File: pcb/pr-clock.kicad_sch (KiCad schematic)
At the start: 6 parts, among them J1 USB_C_Receptacle_USB2.0_16P, U1 TM1637_C2962580, U2 ESP32-C3-WROOM-02, U3 ME6211C33M5, U4 CH340C

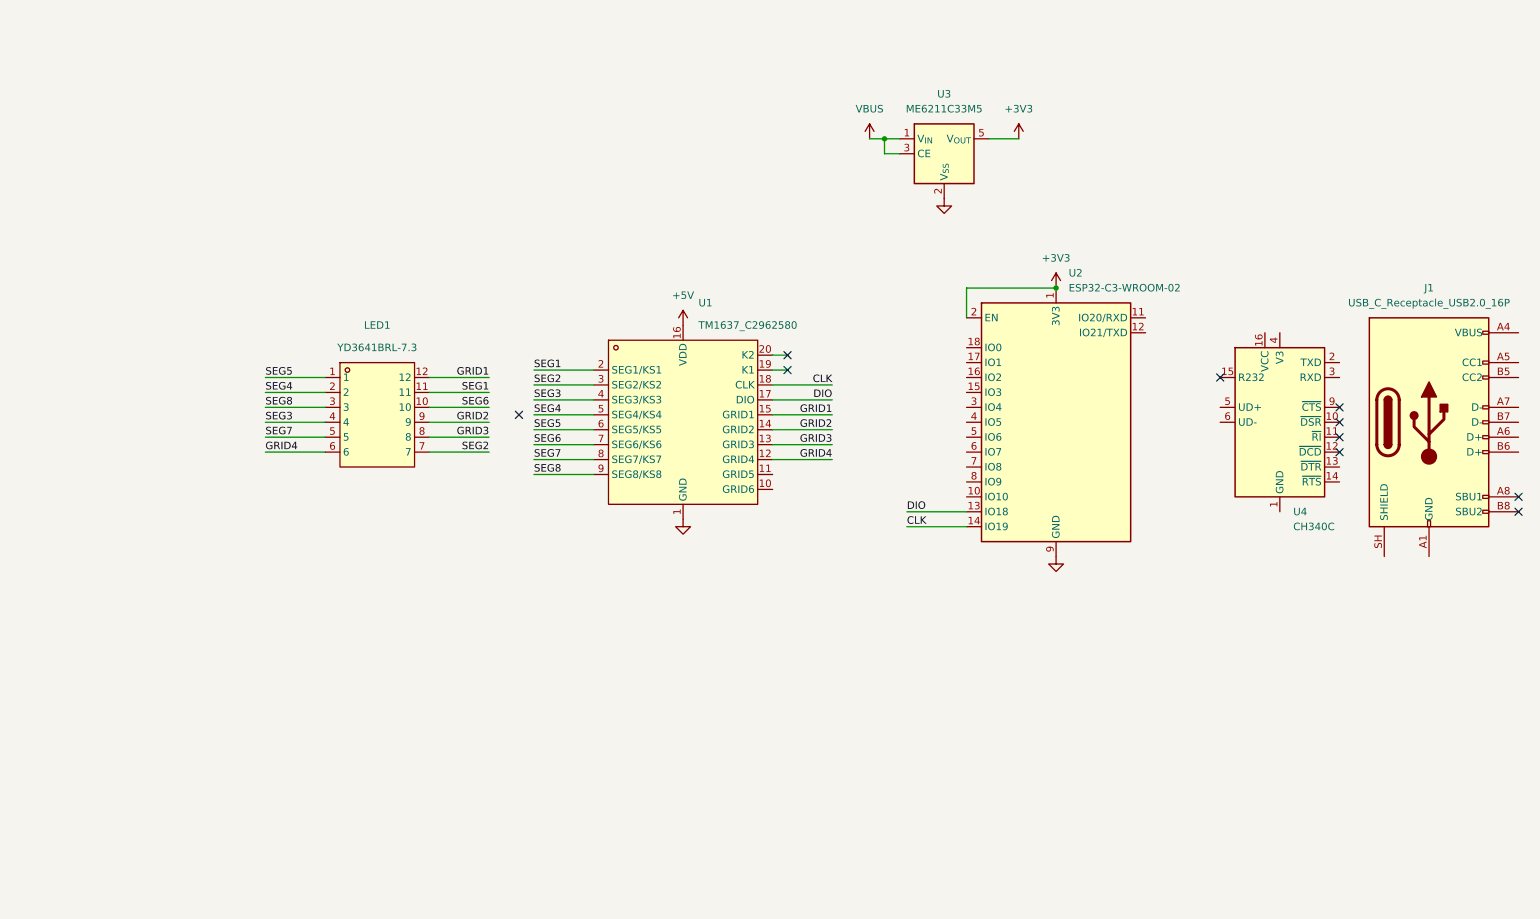
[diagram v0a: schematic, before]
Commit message: yay
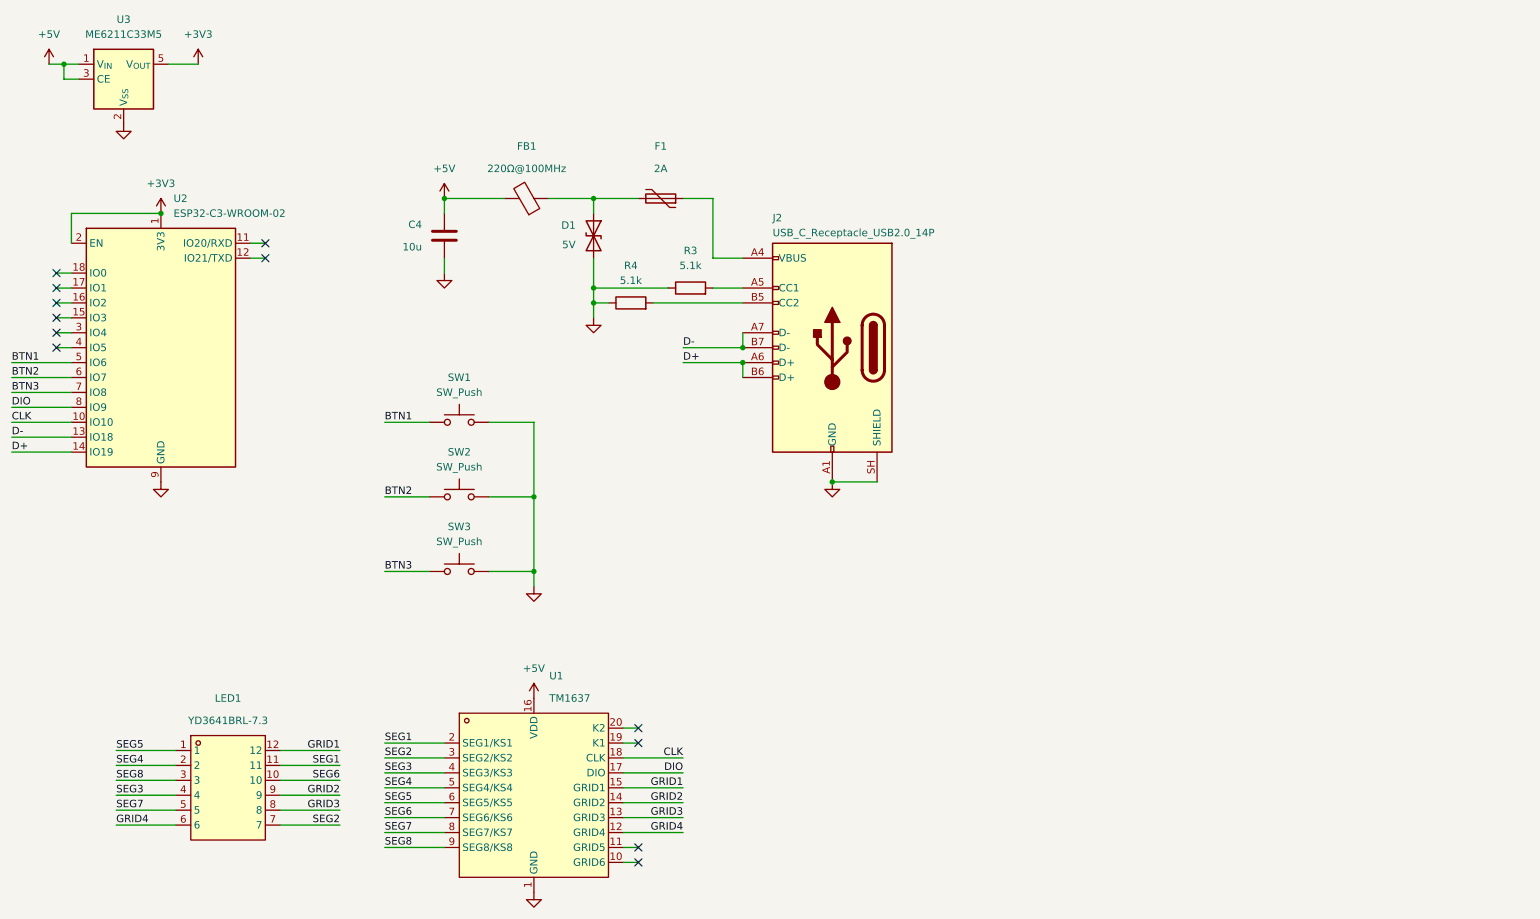
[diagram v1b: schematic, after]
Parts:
- removed J1: USB_C_Receptacle_USB2.0_16P, symbol Connector:USB_C_Receptacle_USB2.0_16P
- removed U4: CH340C, Package_SO:SOIC-16_3.9x9.9mm_P1.27mm, symbol Interface_USB:CH340C
- added C4: 10u, Capacitor_SMD:C_0603_1608Metric, symbol Device:C
- added D1: 5V, Diode_SMD:D_SOD-523, symbol Device:D_TVS
- added F1: 2A, Fuse:Fuse_1206_3216Metric, symbol Device:Polyfuse
- added FB1: 220Ω@100MHz, Resistor_SMD:R_0805_2012Metric_Pad1.20x1.40mm_HandSolder, symbol Device:FerriteBead
- added J2: USB_C_Receptacle_USB2.0_14P, easyeda2kicad:USB-C-SMD_TYPE-C-16PIN-2MD-073, symbol Connector:USB_C_Receptacle_USB2.0_14P
- added R3, R4: 5.1k, Resistor_SMD:R_0603_1608Metric, symbol Device:R
- added SW1, SW2, SW3: SW_Push, toby:SW_Cherry_MX_1.00u_PCB, symbol Switch:SW_Push
- U1: value TM1637_C2962580 -> TM1637
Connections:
- net VBUS is gone; now on net +5V: U3.1 (V_{IN}), U3.3 (CE)
- net +5V: now also C4.1, FB1.2
- net CLK: now also U2.10 (IO10); no longer U2.14 (IO19)
- net DIO: now also U2.8 (IO9); no longer U2.13 (IO18)
- net GND: now also C4.2, D1.2 (A2), J2.A1 (GND), J2.A12 (GND), J2.B1 (GND), J2.B12 (GND), J2.SH (SHIELD), R3.1, R4.1, SW1.2, SW2.2, SW3.2
- net BTN1: now reaches U2.5 (IO6)
- net BTN1: now also SW1.1
- net BTN2: now reaches U2.6 (IO7)
- net BTN2: now also SW2.1
- net BTN3: now reaches U2.7 (IO8)
- net BTN3: now also SW3.1
- new net: J2.B5 (CC2), R4.2
- new net: D1.1 (A1), F1.2, FB1.1
- new net: J2.A5 (CC1), R3.2
- new net: F1.1, J2.A4 (VBUS), J2.A9 (VBUS), J2.B4 (VBUS), J2.B9 (VBUS)
- new net D+: J2.A6 (D+), J2.B6 (D+), U2.14 (IO19)
- new net D-: J2.A7 (D-), J2.B7 (D-), U2.13 (IO18)
- no-connect marks 10 -> 12
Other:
- moved on the sheet: LED1, U1, U2, U3
